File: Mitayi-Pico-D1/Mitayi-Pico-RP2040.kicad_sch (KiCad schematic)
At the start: 56 parts, among them J1 EXP8, J10 GND, J2 USB-C-2.0, J3 Header-1, J4 Header-2, J5 SWD, J6 USB_B_Micro, J7 VBUS, J8 DM, J9 DP, SW1 UK-B0273-SP25Y, SW2 UK-B0273-SP25Y, U1 W25Q32JVSSIQ, U2 MIC5219-3.3YM5, U3 RP2040

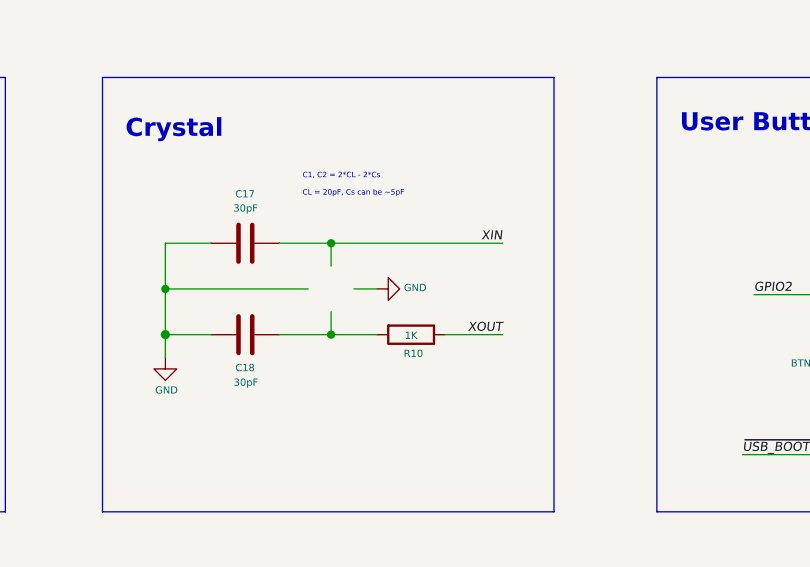
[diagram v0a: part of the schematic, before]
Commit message: Udpated
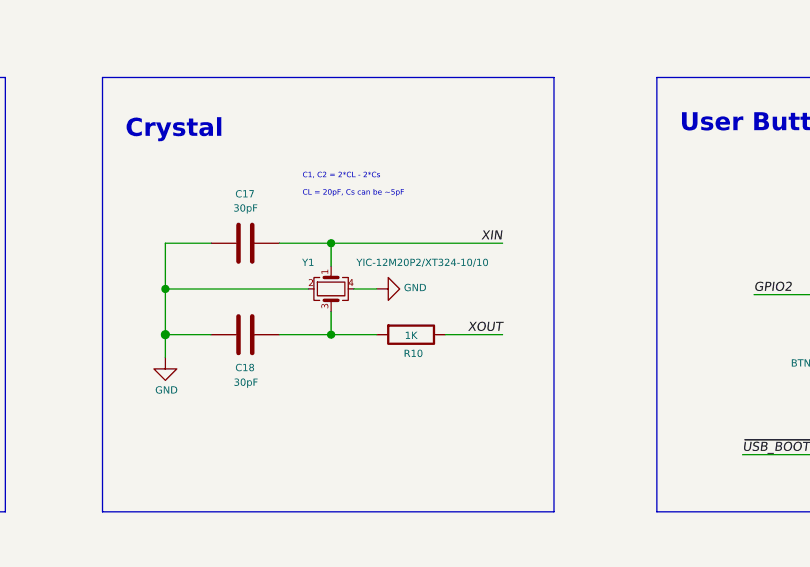
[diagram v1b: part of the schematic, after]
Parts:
- added Y1: YIC-12M20P2/XT324-10/10, Crystal:Crystal_SMD_3225-4Pin_3.2x2.5mm, symbol Device:Crystal_GND24_Small
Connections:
- net GND: now also Y1.2, Y1.4
- net XIN: now also Y1.1
- net at C18.1, R10.2: now also Y1.3
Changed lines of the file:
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@@
+	)
+	(symbol
+		(lib_id "Device:Crystal_GND24_Small")
+		(at 105.41 186.055 270)
+		(unit 1)
+		(exclude_from_sim no)
+		(in_bom yes)
+		(on_board yes)
+		(dnp no)
+		(property "Reference" "Y1"
+			(at 102.87 183.1338 90)
+			(effects
+				(font
+					(size 0.8 0.8)
+				)
+			)
+		)
+		(property "Value" "YIC-12M20P2/XT324-10/10"
+			(at 115.57 183.1338 90)
+			(effects
+				(font
+					(size 0.8 0.8)
+				)
+			)
+		)
+		(property "Footprint" "Crystal:Crystal_SMD_3225-4Pin_3.2x2.5mm"
+			(at 105.41 186.055 0)
+			(hide yes)
+			(effects
+				(font
+					(size 0.8 0.8)
+				)
+			)
+		)
+		(property "Datasheet" ""
+			(at 105.41 186.055 0)
+			(hide yes)
+			(effects
+				(font
+					(size 0.8 0.8)
+				)
+			)
+		)
+		(property "Description" ""
+			(at 105.41 186.055 0)
+			(hide yes)
+			(effects
+				(font
+					(size 1.27 1.27)
+				)
+			)
+		)
+		(property "MFR" "YIC"
+			(at 105.41 186.055 0)
+			(hide yes)
+			(effects
+				(font
+					(size 1.27 1.27)
+				)
+			)
+		)
+		(property "MPN" "YIC-12M20P2/XT324-10/10"
+			(at 105.41 186.055 0)
+			(hide yes)
+			(effects
+				(font
+					(size 1.27 1.27)
+				)
+			)
+		)
+		(property "Name" ""
+			(at 105.41 186.055 0)
+			(hide yes)
+			(effects
+				(font
+					(size 1.27 1.27)
+				)
+			)
+		)
+		(property "Alt MPN" ""
+			(at 105.41 186.055 0)
+			(hide yes)
+			(effects
+				(font
+					(size 1.27 1.27)
+				)
+			)
+		)
+		(pin "1"
+		)
+		(pin "2"
+		)
+		(pin "3"
+		)
+		(pin "4"
+		)
+		(instances
+			(project "Mitayi-Pico-RP2040"
+				(path "/35c47459-45a7-4753-acae-c8b47e7575e1"
+					(reference "Y1")
+					(unit 1)
+				)
+			)
+		)
 	)
 	(symbol
